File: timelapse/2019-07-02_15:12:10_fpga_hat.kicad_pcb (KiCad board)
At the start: 4 copper layers, 65 x 56.5 mm, 90 parts, among them J1 2x20, J2 AudioJack3, J3 Conn_02x06_Top_Bottom, J4 Conn_02x06_Top_Bottom, J5 Conn_02x06_Top_Bottom, J6 Conn_01x02, SW1 PTS815, SW2 PTS815, SW3 PTS815, SW4 PTS815, SW5 PTS815, SW6 PTS815, SW7 PTS815, SW8 PTS815, SW9 PTS815, U1 iCE40-HX8k-BG121, U2 CAT24C32WI, U3 MIC23050-4YML, U4 74LVC2G07, U5 DSC60XX, U6 NCP115ASN330T, U7 W25X40CL, U8 IS61WV25616

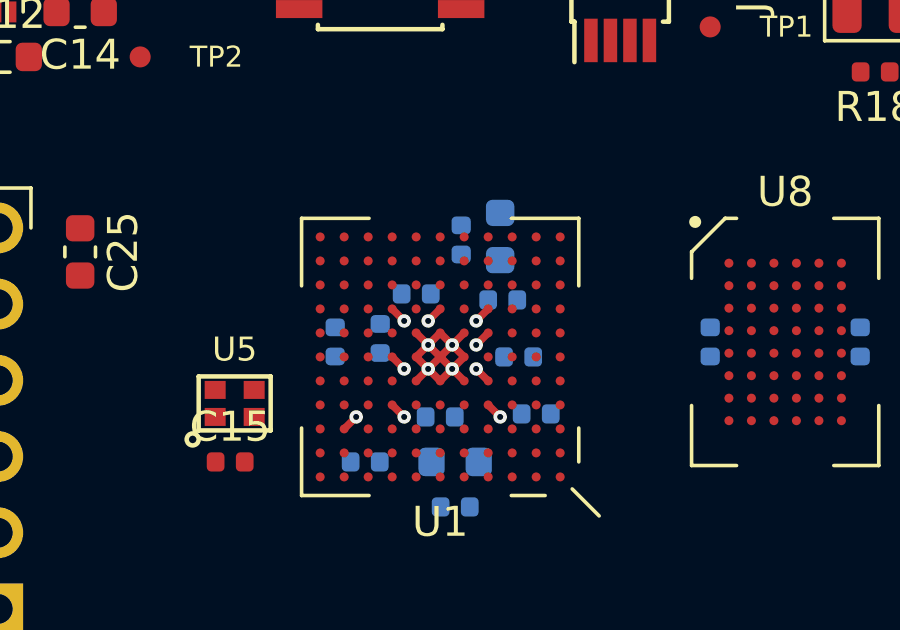
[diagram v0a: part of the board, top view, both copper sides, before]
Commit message: All parts on board
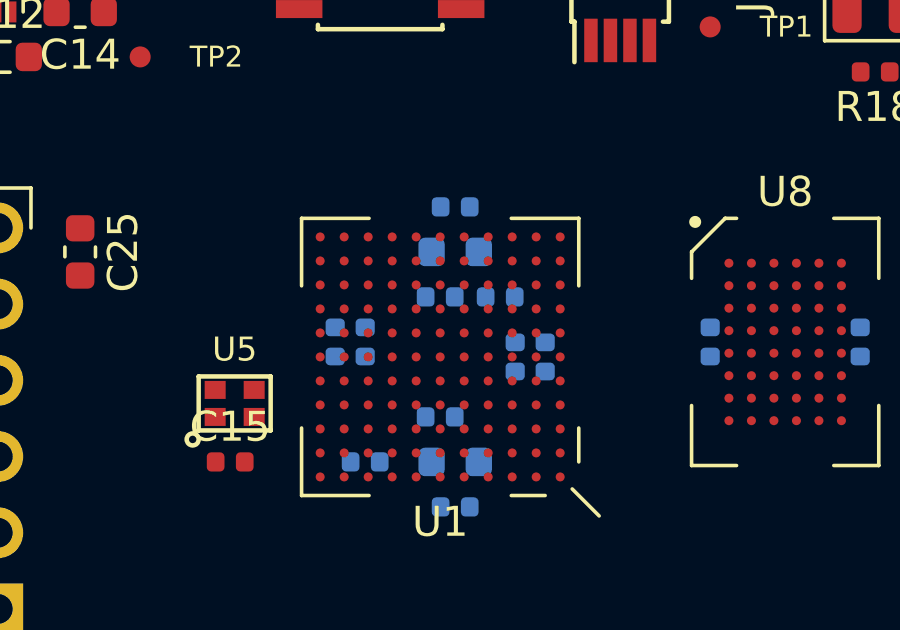
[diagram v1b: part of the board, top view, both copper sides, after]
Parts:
- moved C11 2.80 mm to (134.5, 104.5), turned to 0 degrees
- moved C6 2.09 mm to (132.5, 104.5), turned to 180 degrees
- moved C5 2.02 mm to (135.0, 106.5), turned to 90 degrees
- moved C2 1.59 mm to (133.0, 103.0), turned to 180 degrees
- moved R2 1.12 mm to (133.0, 101.5), turned to 0 degrees
- moved C7 0.88 mm to (136.0, 106.5), turned to 90 degrees
- moved C1 0.51 mm to (130.0, 106.0)
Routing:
- net GND: track 9.05 -> 0.00 mm, vias 4 -> 0
- net +3V3: track 2.83 -> 0.00 mm, vias 5 -> 0
- net +1V2: track 2.26 -> 0.00 mm, vias 4 -> 0
- removed copper zone on In2.Cu, net +5V
